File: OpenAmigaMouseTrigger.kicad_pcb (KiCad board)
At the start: 2 copper layers, 23.9 x 23.9 mm, 8 parts, among them J1 AMIGA_SIGNALS, J2 OUTPUT, J3 POWER, J99 OSHW_LOGO, U1 74LS74

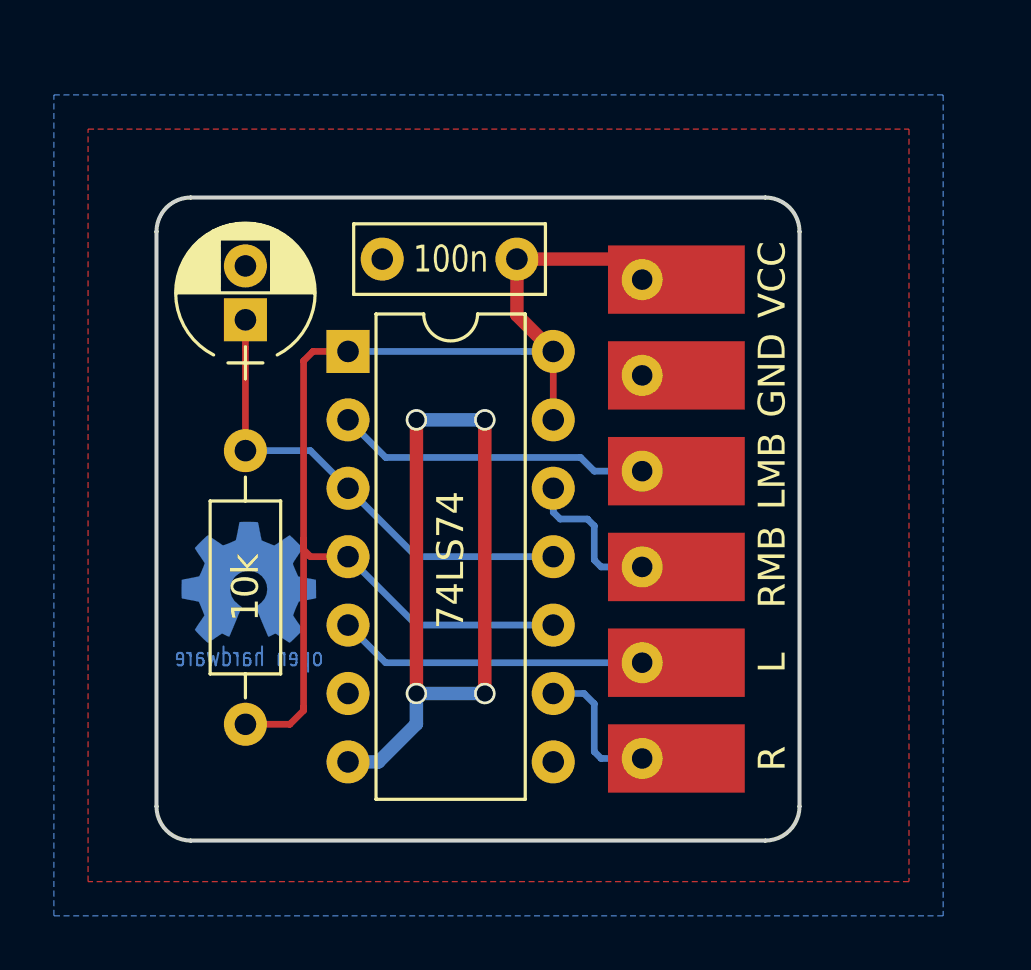
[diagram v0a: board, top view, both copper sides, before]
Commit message: Final touches for V1
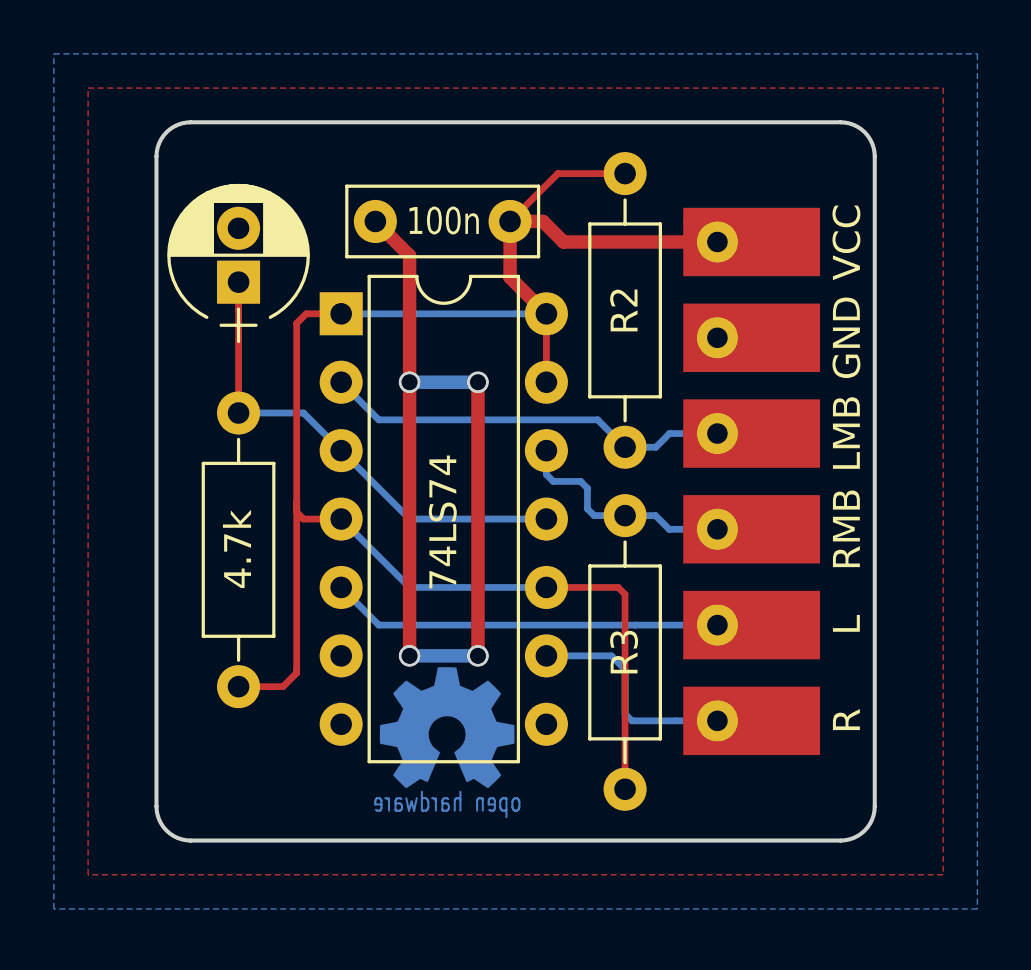
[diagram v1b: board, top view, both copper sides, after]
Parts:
- added R2: 22k, Resistors_THT:R_Axial_DIN0207_L6.3mm_D2.5mm_P10.16mm_Horizontal, F.Cu at (140.6, 95.6)
- added R3: 22k, Resistors_THT:R_Axial_DIN0207_L6.3mm_D2.5mm_P10.16mm_Horizontal, F.Cu at (140.6, 118.5)
- R1: value 10k -> 4.7k
- moved J99 9.13 mm to (134.0, 116.2)
- moved J3 3.12 mm to (145.3, 99.9)
- moved J1 3.12 mm to (145.3, 107.1)
- moved J2 3.12 mm to (145.3, 114.2)
- moved C1 1.42 mm to (126.2, 99.7)
- moved R1 1.42 mm to (126.2, 114.7)
- moved U1 1.42 mm to (130.0, 100.8)
- moved C2 1.42 mm to (136.3, 97.4)
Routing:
- net VCC: track 46.9 -> 66.3 mm
- net Net-(J1-Pad1): track 11.7 -> 14.9 mm
- net Net-(J2-Pad1): track 11.5 -> 14.5 mm
- net Net-(J2-Pad2): track 5.34 -> 8.06 mm
- net Net-(J1-Pad2): track 5.78 -> 8.27 mm
- net GND: track 29.7 -> 31.9 mm
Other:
- board size 23.9 x 23.9 mm -> 26.7 x 26.7 mm
- board text added: "V1"

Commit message: V2 is ready
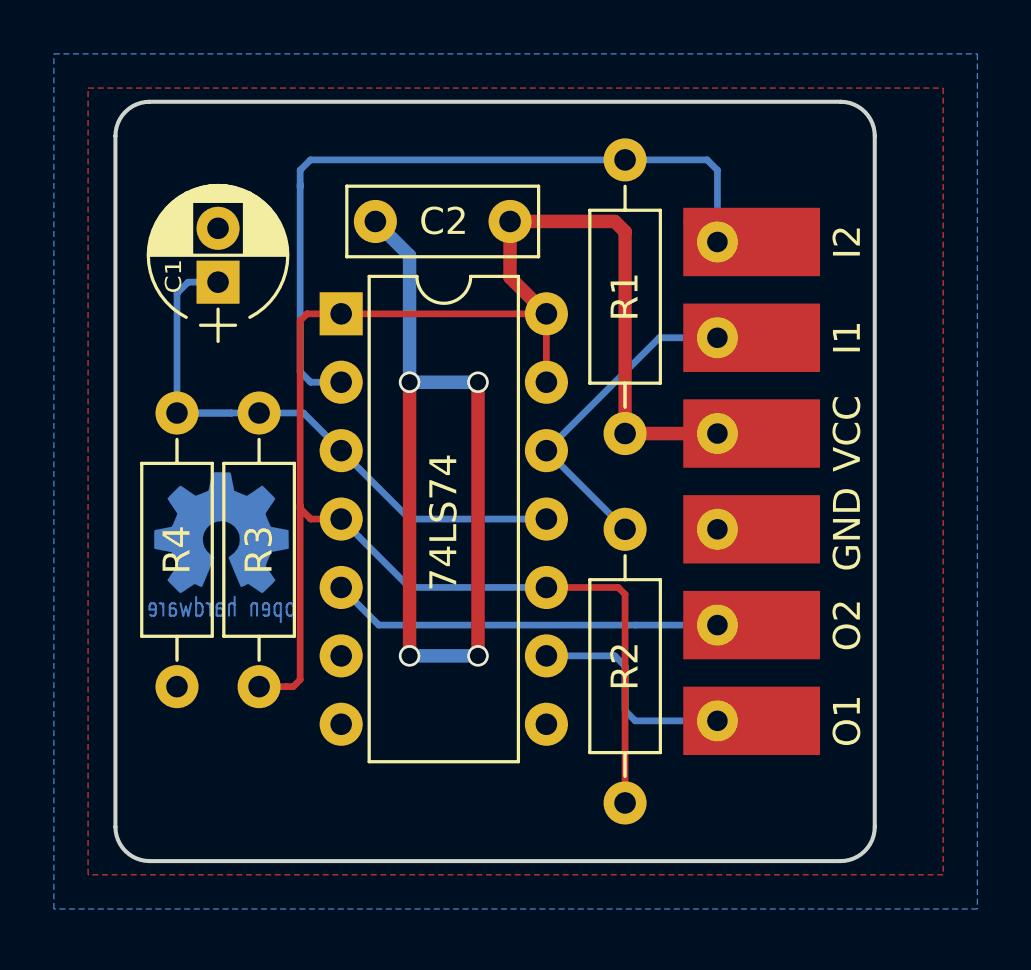
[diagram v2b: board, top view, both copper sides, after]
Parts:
- added R4: 330k, Resistors_THT:R_Axial_DIN0207_L6.3mm_D2.5mm_P10.16mm_Horizontal, F.Cu at (124.0, 104.5)
- J1: value AMIGA_SIGNALS -> INPUT_SIGNALS
- moved J99 11.1 mm to (125.6, 109.0)
- moved R1 9.65 mm to (140.6, 105.3), turned to 90 degrees
- moved J1 7.11 mm to (145.3, 99.9)
- moved J3 7.11 mm to (145.3, 107.1)
- moved C1 0.76 mm to (125.5, 99.7)
- moved R3 0.76 mm to (127.0, 114.7)
- moved R2 0.51 mm to (140.6, 119.0)
- renumbered R2 to R1, R3 to R2, R1 to R3
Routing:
- net Net-(J1-Pad1): track 14.9 -> 28.8 mm
- net Net-(C1-Pad1): track 17.9 -> 23.3 mm
- net Net-(J1-Pad2): track 8.27 -> 12.7 mm
- net VCC: track 66.3 -> 67.9 mm
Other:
- board size 26.7 x 26.7 mm -> 28.2 x 28.2 mm
- board text added: "I1"
- board text added: "I2"
- board text added: "O1"
- board text added: "O2"
- board text added: "V2"
- board text removed: "L"
- board text removed: "LMB"
- board text removed: "R"
- board text removed: "RMB"
- board text removed: "V1"
